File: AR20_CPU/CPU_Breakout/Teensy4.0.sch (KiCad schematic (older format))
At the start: 15 parts, among them SW1 SW_SPST

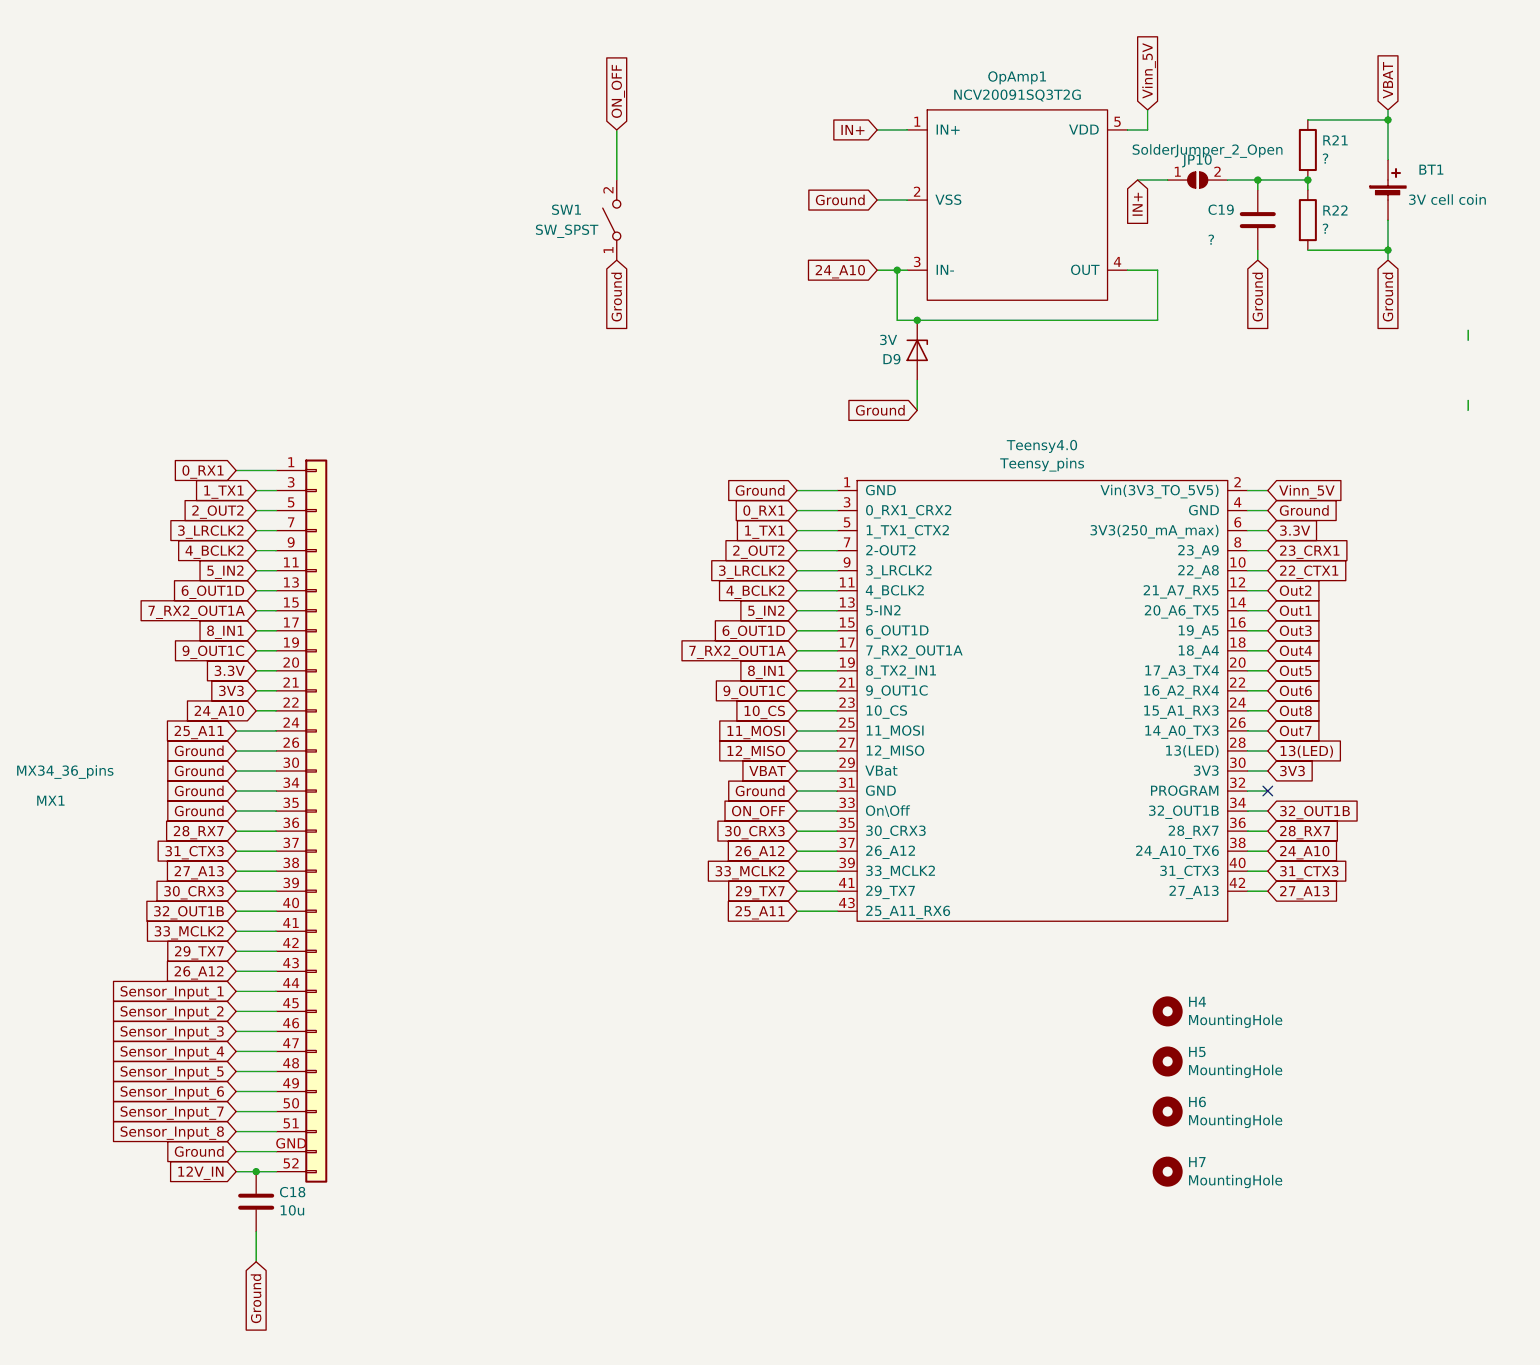
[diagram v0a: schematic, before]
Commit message: E
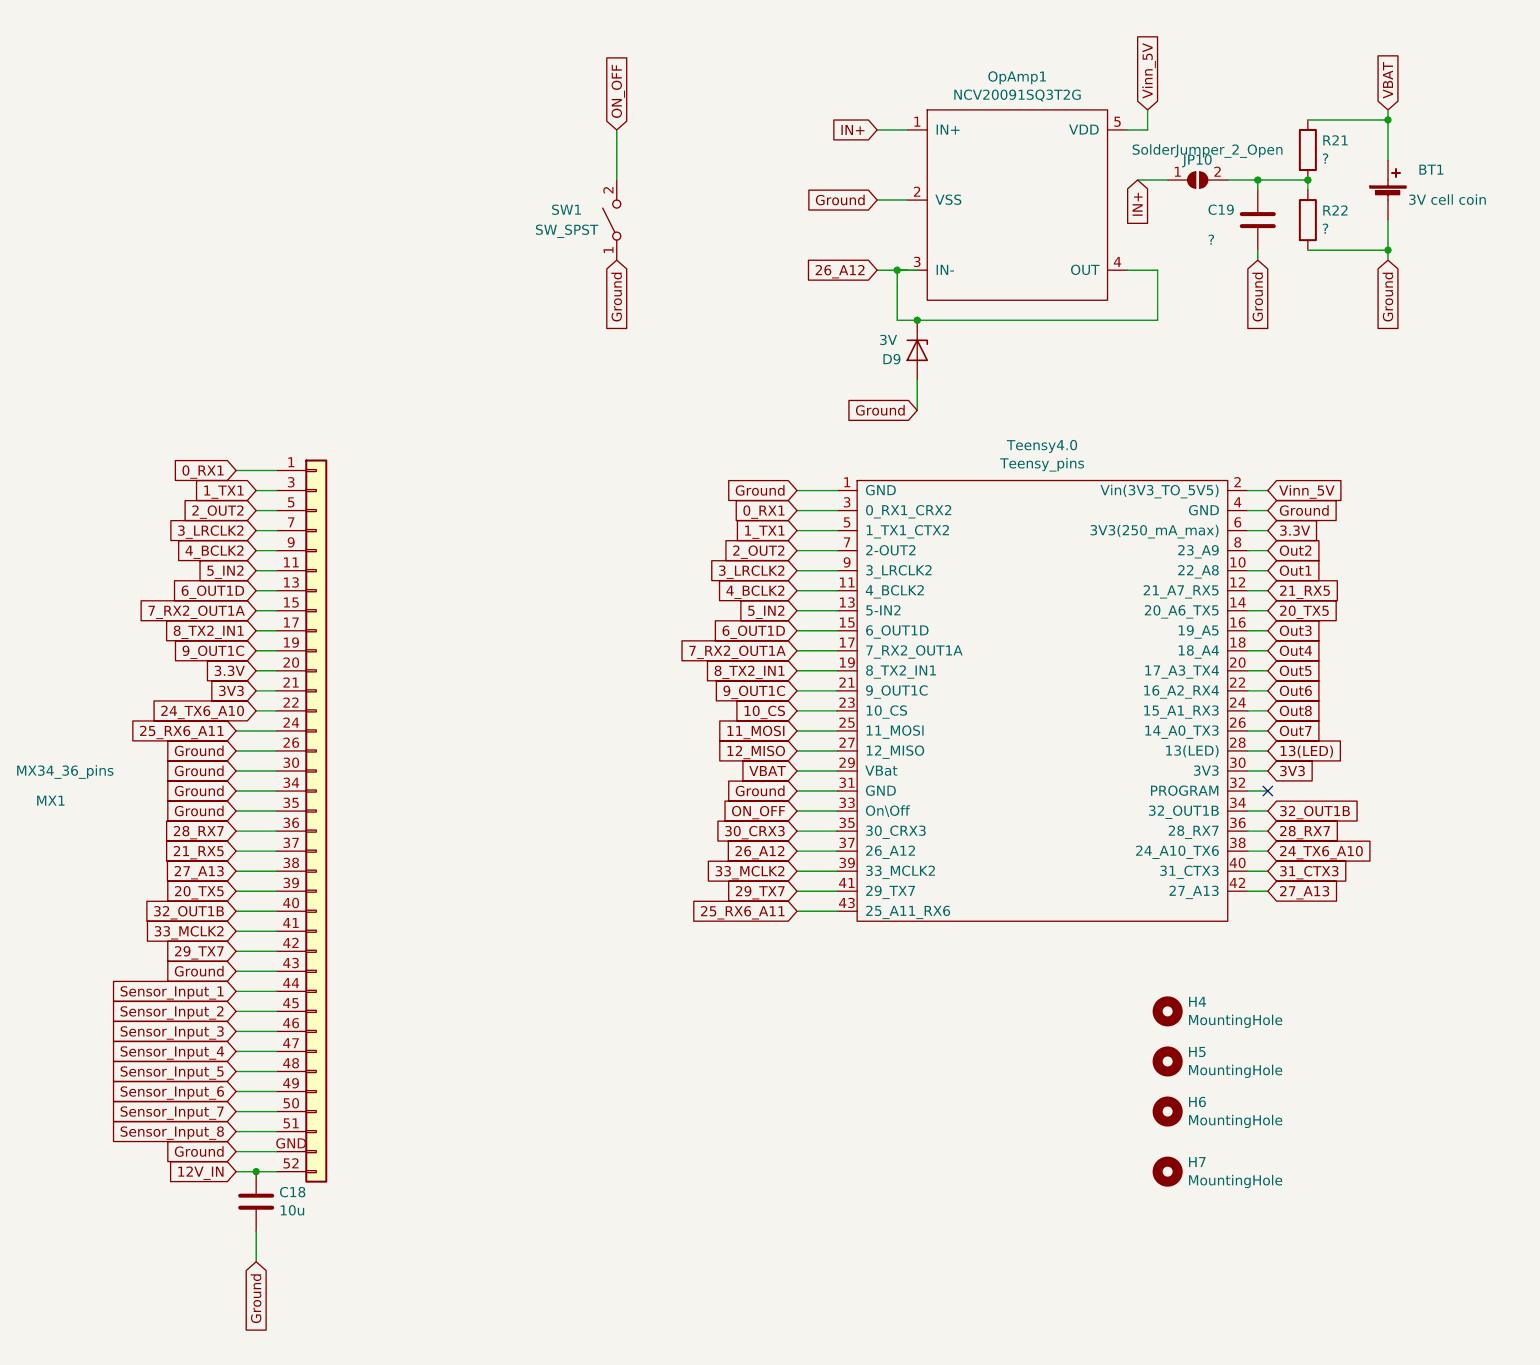
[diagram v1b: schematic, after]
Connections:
- net 22_CTX1 is gone; now on net Out1: Teensy4.0.10 (22_A8)
- net 23_CRX1 is gone; now on net Out2: Teensy4.0.8 (23_A9)
- net 26_A12: now also D9.1 (K), OpAmp1.3 (IN-), OpAmp1.4 (OUT); no longer MX1.43 (Pin_43)
- net 30_CRX3: no longer MX1.39 (Pin_39)
- net 31_CTX3: no longer MX1.37 (Pin_37)
- net Ground: now also MX1.43 (Pin_43)
- net Out1: no longer Teensy4.0.14 (20_A6_TX5)
- net Out2: no longer Teensy4.0.12 (21_A7_RX5)
- removed net 24_A10: D9.1 (K), MX1.22 (Pin_22), OpAmp1.3 (IN-), OpAmp1.4 (OUT), Teensy4.0.38 (24_A10_TX6)
- net 25_A11 renamed 25_RX6_A11
- net 8_IN1 renamed 8_TX2_IN1
- new net 20_TX5: MX1.39 (Pin_39), Teensy4.0.14 (20_A6_TX5)
- new net 21_RX5: MX1.37 (Pin_37), Teensy4.0.12 (21_A7_RX5)
- new net 24_TX6_A10: MX1.22 (Pin_22), Teensy4.0.38 (24_A10_TX6)
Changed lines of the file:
@@
 Text GLabel 9550 3500 2    50   Input ~ 0
 Out3
-Text GLabel 9550 3400 2    50   Input ~ 0
+Text GLabel 9550 3200 2    50   Input ~ 0
 Out1
-Text GLabel 9550 3300 2    50   Input ~ 0
+Text GLabel 9550 3100 2    50   Input ~ 0
 Out2
 Text GLabel 9550 3600 2    50   Input ~ 0
@@
 26_A12
 Text GLabel 9550 4600 2    50   Input ~ 0
-24_A10
+24_TX6_A10
 Text GLabel 9550 4200 2    50   Input ~ 0
 3V3
@@
 Text GLabel 9550 2800 2    50   Input ~ 0
 Vinn_5V
-Text GLabel 9550 3100 2    50   Input ~ 0
-23_CRX1
-Text GLabel 9550 3200 2    50   Input ~ 0
-22_CTX1
+Text GLabel 9550 3300 2    50   Input ~ 0
+21_RX5
+Text GLabel 9550 3400 2    50   Input ~ 0
+20_TX5
 $Comp
 L BreakoutBoardTeensy:Teensy_pins Teensy4.?
@@
 27_A13
 Text GLabel 7200 4900 0    50   Input ~ 0
-25_A11
+25_RX6_A11
 Text GLabel 7200 3800 0    50   Input ~ 0
 9_OUT1C
 Text GLabel 7200 3700 0    50   Input ~ 0
-8_IN1
+8_TX2_IN1
 Text GLabel 7200 3600 0    50   Input ~ 0
 7_RX2_OUT1A
@@
 Wire Wire Line
 	4600 3900 4500 3900
-Text GLabel 4500 3900 0    50   Input ~ 0
-24_A10
-Text GLabel 4400 5200 0    50   Input ~ 0
-26_A12
 Text GLabel 4400 4500 0    50   Input ~ 0
 28_RX7
 Text GLabel 4400 5000 0    50   Input ~ 0
 33_MCLK2
-Text GLabel 4400 4600 0    50   Input ~ 0
-31_CTX3
 Text GLabel 4400 5100 0    50   Input ~ 0
 29_TX7
 Text GLabel 4400 4700 0    50   Input ~ 0
 27_A13
-Text GLabel 4400 4000 0    50   Input ~ 0
-25_A11
 Text GLabel 4500 3600 0    50   Input ~ 0
 9_OUT1C
-Text GLabel 4500 3500 0    50   Input ~ 0
-8_IN1
 Text GLabel 4500 3400 0    50   Input ~ 0
 7_RX2_OUT1A
@@
 Wire Wire Line
 	4600 5800 4400 5800
-Text GLabel 4400 4800 0    50   Input ~ 0
-30_CRX3
 Text GLabel 4400 4900 0    50   Input ~ 0
 32_OUT1B
@@
 Wire Wire Line
 	9050 1250 8900 1250
-Text GLabel 7600 1700 0    50   Input ~ 0
-24_A10
 $Comp
 L Device:C C19
@@
 Wire Wire Line
 	7700 1700 7750 1700
-Wire Wire Line
-	10550 2050 10550 2000
-Wire Wire Line
-	10550 2400 10550 2350
 $Comp
 L Device:D_Zener D?
@@
 Wire Wire Line
 	7800 2400 7800 2250
+Text GLabel 4400 4600 0    50   Input ~ 0
+21_RX5
+Text GLabel 4400 4800 0    50   Input ~ 0
+20_TX5
+Text GLabel 4500 3500 0    50   Input ~ 0
+8_TX2_IN1
+Text GLabel 4400 4000 0    50   Input ~ 0
+25_RX6_A11
+Text GLabel 4500 3900 0    50   Input ~ 0
+24_TX6_A10
+Text GLabel 4400 5200 0    50   Input ~ 0
+Ground
+Text GLabel 7600 1700 0    50   Input ~ 0
+26_A12
+Wire Wire Line
+	7800 1700 7700 1700
 $EndSCHEMATC

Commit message: E2
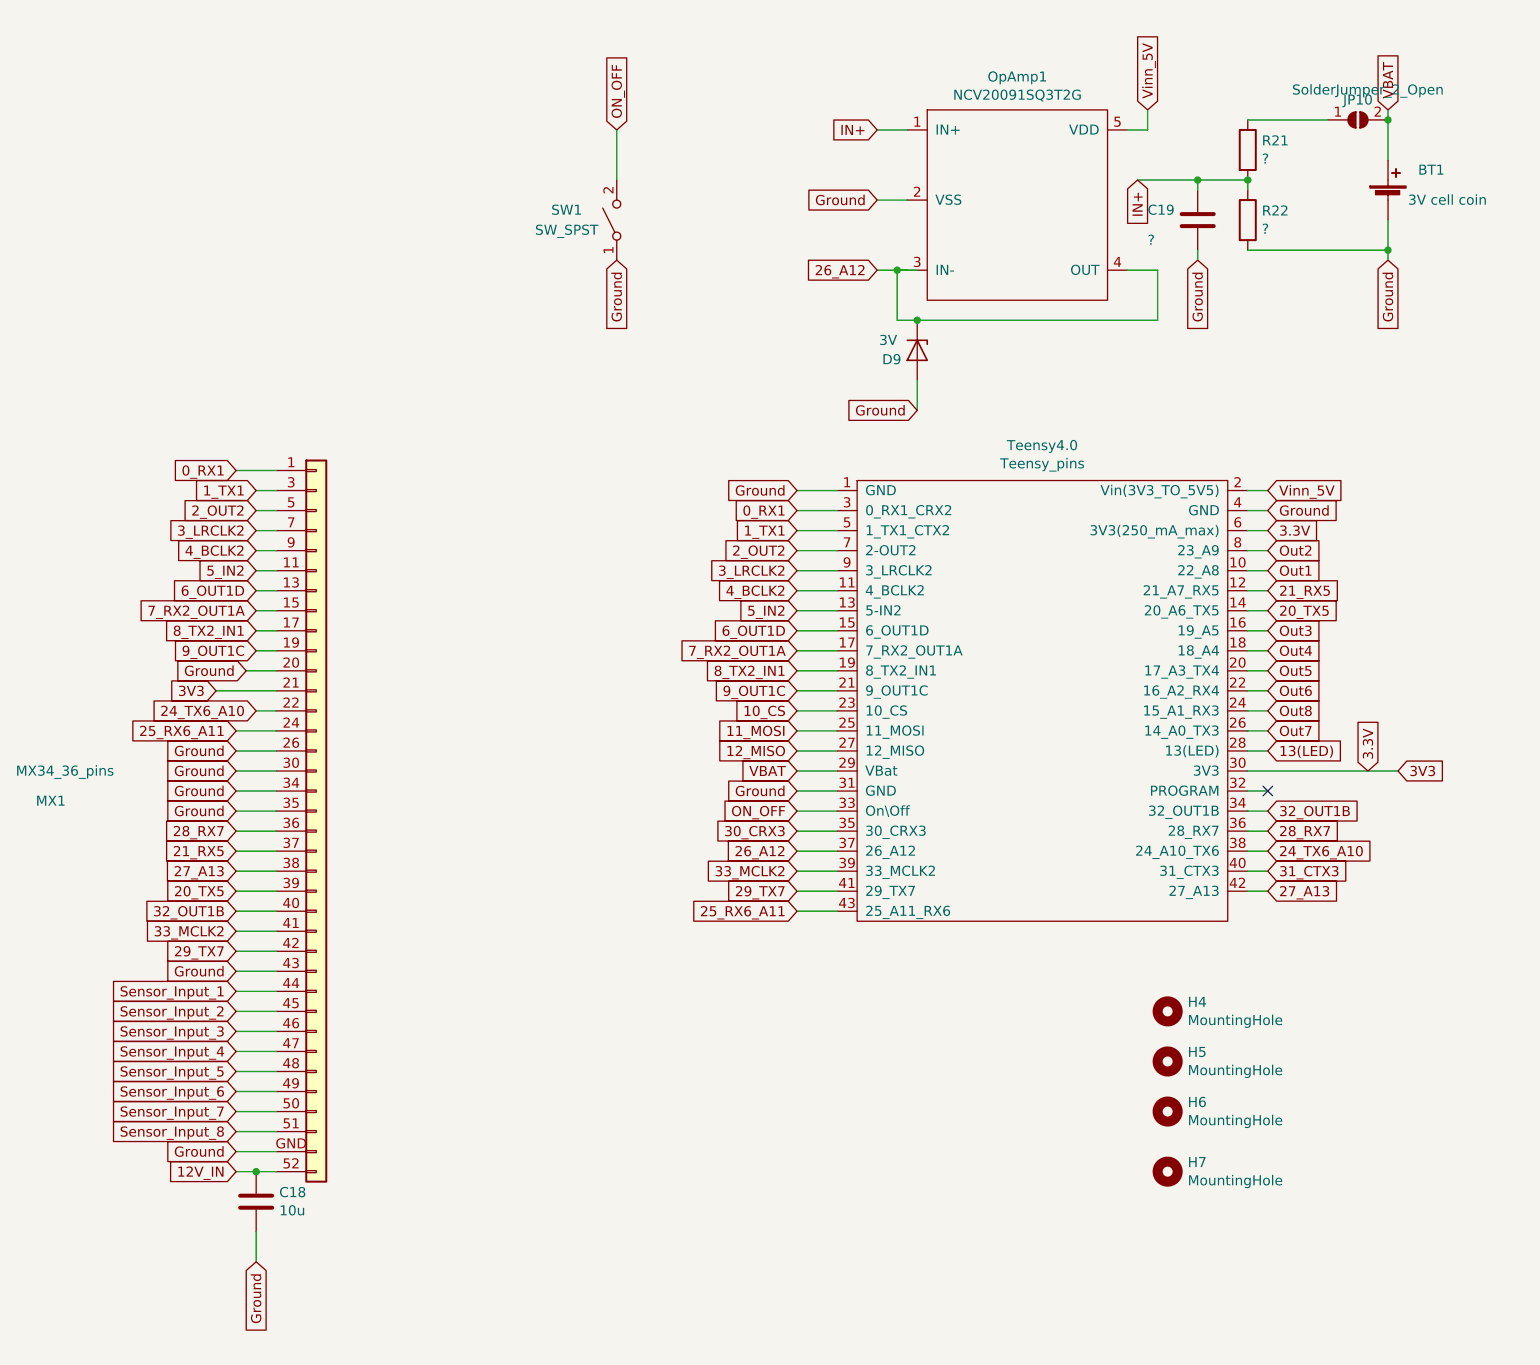
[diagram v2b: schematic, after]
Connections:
- net 3V3 is gone; now on net 3.3V: MX1.21 (Pin_21), Teensy4.0.30 (3V3)
- net 3.3V: no longer MX1.20 (Pin_20)
- net Ground: now also MX1.20 (Pin_20)
- net IN+: now also C19.1, R21.2, R22.1; no longer JP10.1 (A)
- net VBAT: now also JP10.2 (B); no longer R21.1
- new net: JP10.1 (A), R21.1
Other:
- moved on the sheet: C19, JP10, R21, R22
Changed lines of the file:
@@
 Text GLabel 9550 4600 2    50   Input ~ 0
 24_TX6_A10
-Text GLabel 9550 4200 2    50   Input ~ 0
+Text GLabel 10200 4200 2    50   Input ~ 0
 3V3
 Text GLabel 9550 3000 2    50   Input ~ 0
@@
 	9450 4000 9550 4000
 Wire Wire Line
-	9450 4200 9550 4200
-Wire Wire Line
 	9450 4300 9550 4300
 Wire Wire Line
@@
 	4600 3600 4500 3600
 Wire Wire Line
-	4600 3700 4500 3700
-Wire Wire Line
-	4600 3800 4500 3800
-Wire Wire Line
 	4600 3900 4500 3900
 Text GLabel 4400 4500 0    50   Input ~ 0
@@
 Text GLabel 4400 4900 0    50   Input ~ 0
 32_OUT1B
-Text GLabel 4500 3800 0    50   Input ~ 0
+Text GLabel 4300 3800 0    50   Input ~ 0
 3V3
 Wire Wire Line
@@
 Text GLabel 4400 4400 0    50   Input ~ 0
 Ground
-Text GLabel 4500 3700 0    50   Input ~ 0
-3.3V
 $Comp
 L Device:R R21
 U 1 1 5DE96DA3
-P 9750 1100
-F 0 "R21" H 9820 1146 50  0000 L CNN
-F 1 "?" H 9820 1055 50  0000 L CNN
-F 2 "Resistor_SMD:R_0603_1608Metric" V 9680 1100 50  0001 C CNN
-F 3 "~" H 9750 1100 50  0001 C CNN
-	1    9750 1100
+P 9450 1100
+F 0 "R21" H 9520 1146 50  0000 L CNN
+F 1 "?" H 9520 1055 50  0000 L CNN
+F 2 "Resistor_SMD:R_0603_1608Metric" V 9380 1100 50  0001 C CNN
+F 3 "~" H 9450 1100 50  0001 C CNN
+	1    9450 1100
 	1    0    0    -1
 $EndComp
@@
 L Device:R R22
 U 1 1 5DE9741A
-P 9750 1450
-F 0 "R22" H 9820 1496 50  0000 L CNN
-F 1 "?" H 9820 1405 50  0000 L CNN
-F 2 "Resistor_SMD:R_0603_1608Metric" V 9680 1450 50  0001 C CNN
-F 3 "~" H 9750 1450 50  0001 C CNN
-	1    9750 1450
+P 9450 1450
+F 0 "R22" H 9520 1496 50  0000 L CNN
+F 1 "?" H 9520 1405 50  0000 L CNN
+F 2 "Resistor_SMD:R_0603_1608Metric" V 9380 1450 50  0001 C CNN
+F 3 "~" H 9450 1450 50  0001 C CNN
+	1    9450 1450
 	1    0    0    -1
 $EndComp
 Wire Wire Line
-	10150 1150 10150 950
+	9450 1300 9450 1250
 Wire Wire Line
-	10150 1450 10150 1600
-Wire Wire Line
-	9750 1300 9750 1250
-Wire Wire Line
-	9750 950  10150 950
-Connection ~ 10150 950
-Wire Wire Line
-	10150 950  10150 900
-Wire Wire Line
-	9750 1600 10150 1600
-Connection ~ 10150 1600
-Wire Wire Line
-	10150 1600 10150 1650
-Connection ~ 9750 1250
+	9450 950  9850 950
+Connection ~ 9450 1250
 $Comp
 L Jumper:SolderJumper_2_Open JP10
 U 1 1 5DEBD2EA
-P 9200 1250
-F 0 "JP10" H 9200 1350 50  0000 C CNN
-F 1 "SolderJumper_2_Open" H 9250 1400 50  0000 C CNN
-F 2 "Jumper:SolderJumper-2_P1.3mm_Open_RoundedPad1.0x1.5mm" H 9200 1250 50  0001 C CNN
-F 3 "~" H 9200 1250 50  0001 C CNN
-	1    9200 1250
+P 10000 950
+F 0 "JP10" H 10000 1050 50  0000 C CNN
+F 1 "SolderJumper_2_Open" H 10050 1100 50  0000 C CNN
+F 2 "Jumper:SolderJumper-2_P1.3mm_Open_RoundedPad1.0x1.5mm" H 10000 950 50  0001 C CNN
+F 3 "~" H 10000 950 50  0001 C CNN
+	1    10000 950
 	1    0    0    -1
 $EndComp
-Wire Wire Line
-	9050 1250 8900 1250
 $Comp
 L Device:C C19
 U 1 1 5DEC35AF
-P 9500 1450
-F 0 "C19" H 9250 1500 50  0000 L CNN
-F 1 "?" H 9250 1350 50  0000 L CNN
-F 2 "Capacitor_SMD:C_0603_1608Metric" H 9538 1300 50  0001 C CNN
-F 3 "~" H 9500 1450 50  0001 C CNN
-	1    9500 1450
+P 9200 1450
+F 0 "C19" H 8950 1500 50  0000 L CNN
+F 1 "?" H 8950 1350 50  0000 L CNN
+F 2 "Capacitor_SMD:C_0603_1608Metric" H 9238 1300 50  0001 C CNN
+F 3 "~" H 9200 1450 50  0001 C CNN
+	1    9200 1450
 	1    0    0    -1
 $EndComp
 Wire Wire Line
-	9500 1300 9500 1250
-Connection ~ 9500 1250
-Wire Wire Line
-	9500 1250 9350 1250
+	9200 1300 9200 1250
+Connection ~ 9200 1250
 Wire Wire Line
-	9500 1250 9750 1250
-Text GLabel 9500 1650 3    50   Input ~ 0
+	9200 1250 9450 1250
+Text GLabel 9200 1650 3    50   Input ~ 0
 Ground
 Wire Wire Line
-	9500 1600 9500 1650
+	9200 1600 9200 1650
 Text GLabel 8950 900  1    50   Input ~ 0
 Vinn_5V
@@
 Wire Wire Line
 	7800 1700 7700 1700
+Wire Wire Line
+	4300 3800 4600 3800
+Text GLabel 4450 3700 0    50   Input ~ 0
+Ground
+Wire Wire Line
+	4450 3700 4600 3700
+Wire Wire Line
+	10150 900  10150 950
+Wire Wire Line
+	10150 1450 10150 1600
+Wire Wire Line
+	8900 1250 9200 1250
+Connection ~ 10150 950
+Wire Wire Line
+	10150 950  10150 1150
+Wire Wire Line
+	9450 1600 10150 1600
+Connection ~ 10150 1600
+Wire Wire Line
+	10150 1600 10150 1650
+Text GLabel 10050 4200 1    50   Input ~ 0
+3.3V
+Wire Wire Line
+	9450 4200 10200 4200
 $EndSCHEMATC
